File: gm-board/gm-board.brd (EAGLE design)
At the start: 56.8 x 31.1 mm, 46 parts, among them IC1 MCP1700TT, IC2 ZXCT1109, IC3 STM32F030F4, J1 HV_GEN-HOLE, J3 SWD_SHROUD, X1 PKM13EPYH

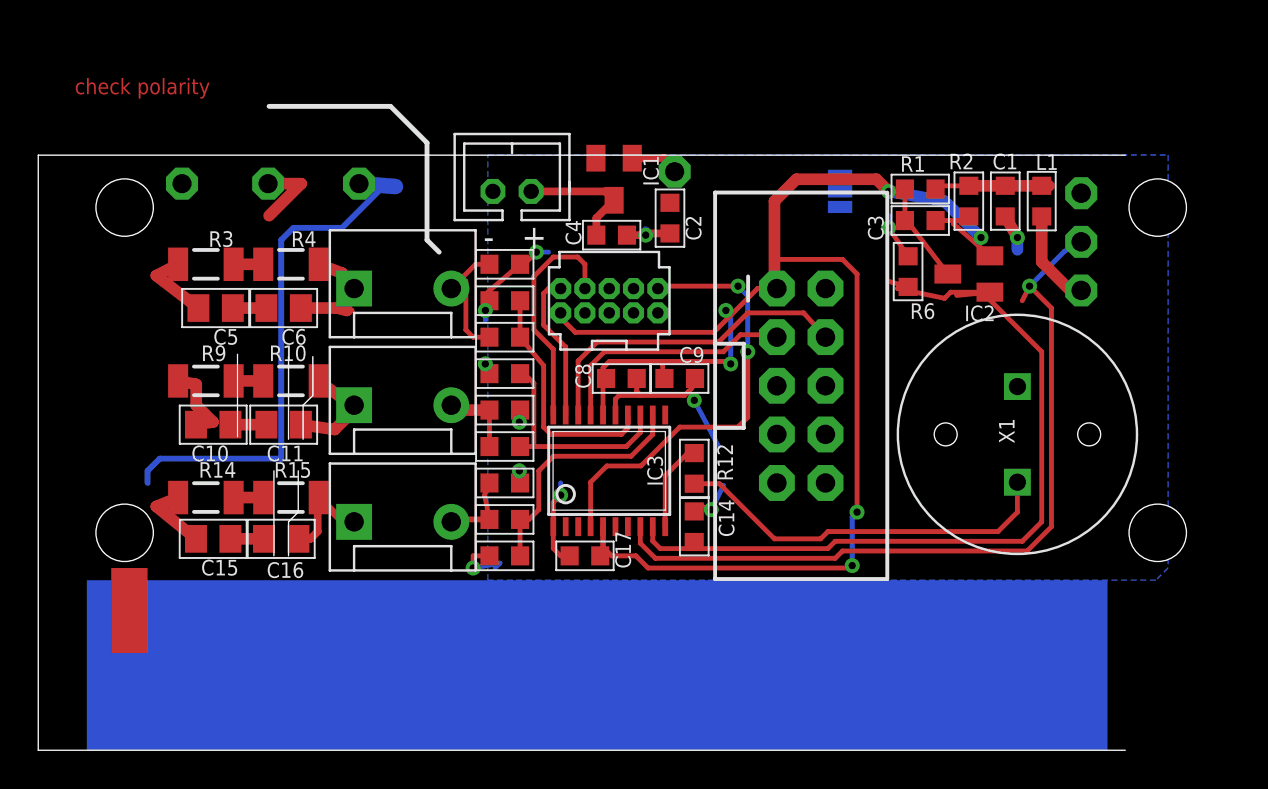
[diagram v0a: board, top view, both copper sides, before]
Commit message: gettuing there...
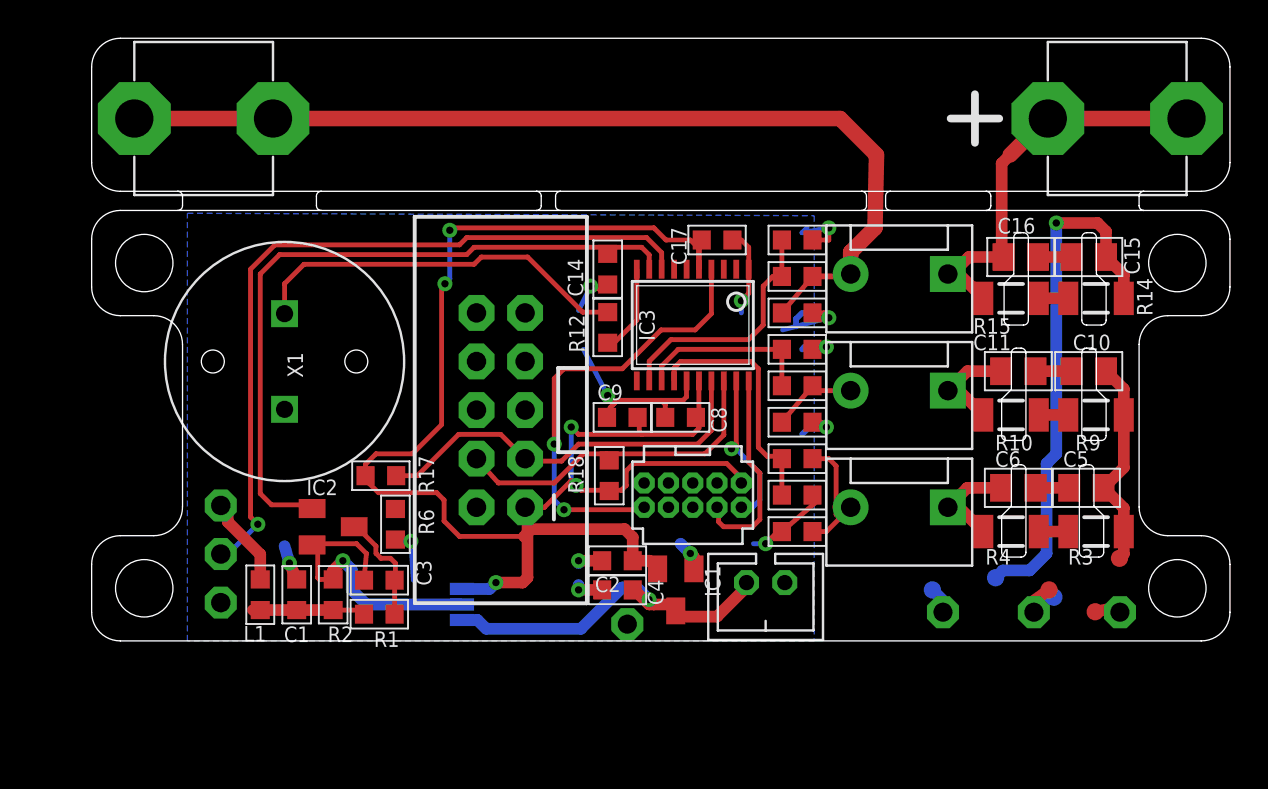
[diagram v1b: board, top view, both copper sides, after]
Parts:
- added R17, R18: (no value), passives-7351:R0603-N
- added TP1, TP2, TP3, TP4, TP5, TP6: TPTP09R, testpad:TP09R
- added X2: GM-TUBE, Mine:GM-TUBE
- J2: device dtb:JST-2-TH -> dtb:JST-2-TH-NOTEXT
- moved J1 55.2 mm to (5.00, 0.00), turned to 0 degrees
- moved R3 48.6 mm to (52.8, 5.71), turned to 0 degrees
- moved C15 48.1 mm to (52.4, 20.1), turned to 0 degrees
- moved R14 47.7 mm to (52.8, 17.9), turned to 0 degrees
- moved R9 46.6 mm to (52.8, 11.8), turned to 0 degrees
- moved C5 46.5 mm to (52.2, 8.00), turned to 0 degrees
- moved C10 45.9 mm to (52.4, 14.1), turned to 0 degrees
- moved L1 45.7 mm to (9.06, 2.41), turned to 90 degrees
- moved C1 42.4 mm to (11.0, 2.41), turned to 270 degrees
- moved C16 41.4 mm to (48.8, 20.1), turned to 0 degrees
- moved R4 40.1 mm to (48.3, 5.71), turned to 0 degrees
- moved C6 39.5 mm to (48.7, 8.00), turned to 0 degrees
- moved R2 39.1 mm to (12.9, 2.41), turned to 90 degrees
- moved R15 39.1 mm to (48.3, 17.9), turned to 0 degrees
- moved C11 38.5 mm to (48.7, 14.1), turned to 0 degrees
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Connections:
- new net N$10: J1.HV3, TP1.TP
- new net N$12: J1.HV2, TP2.TP, TP6.TP
- new net N$13: J1.HV1, TP3.TP
- net +3V3: now also R17.2, R18.2
- net N$1: now also X2.B1, X2.B2
- net N$20: now also TP4.TP; no longer J1.HV2
- net N$3: now also X2.A1, X2.A2
- net N$8: now also TP5.TP; no longer J1.HV1
- net SCL: now also R17.1
- net SDA: now also R18.1
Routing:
- net N$1: track 4.45 -> 51.7 mm
- net N$3: track 5.34 -> 21.2 mm
- net VIN: track 6.73 -> 18.9 mm, vias 0 -> 1
- net N$11: track 4.61 -> 16.3 mm, vias 0 -> 1
- net SCL: track 13.0 -> 21.2 mm
- net HV_CURRENT: track 44.5 -> 36.7 mm
- net +3V3: track 79.6 -> 86.0 mm, vias 6 -> 5
- net N$8: track 32.3 -> 27.3 mm, vias 0 -> 1
- net GND: track 38.3 -> 42.8 mm, vias 12 -> 13
- net N$12: track 0.00 -> 3.27 mm
- net TIM17_CH1: track 11.7 -> 9.33 mm
- net N$10: track 0.00 -> 2.19 mm
- net SWCLK: track 12.2 -> 10.7 mm
- net HV_SHDN: track 40.8 -> 39.4 mm
- net N$13: track 0.00 -> 1.40 mm
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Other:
- board size 56.8 x 31.1 mm -> 59.5 x 31.5 mm
- board text removed: "check polarity"
